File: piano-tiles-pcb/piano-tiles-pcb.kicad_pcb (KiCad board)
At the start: 2 copper layers, 72 x 52 mm, 18 parts, among them J1 Conn_01x05, J2 Conn_01x05, SW1 SW_SPST, SW2 SW_SPST, SW3 SW_SPST, SW4 SW_SPST, SW5 SW_SPDT

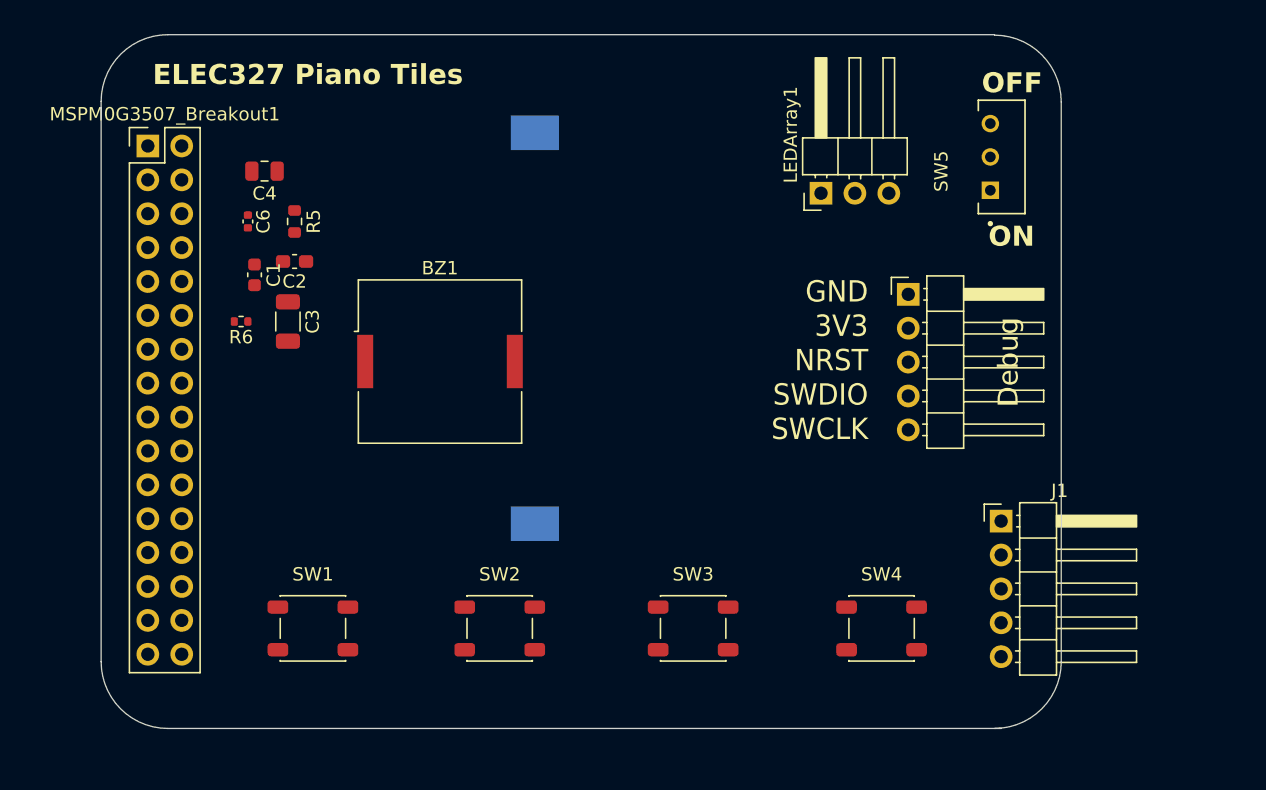
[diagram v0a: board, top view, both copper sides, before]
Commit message: first order
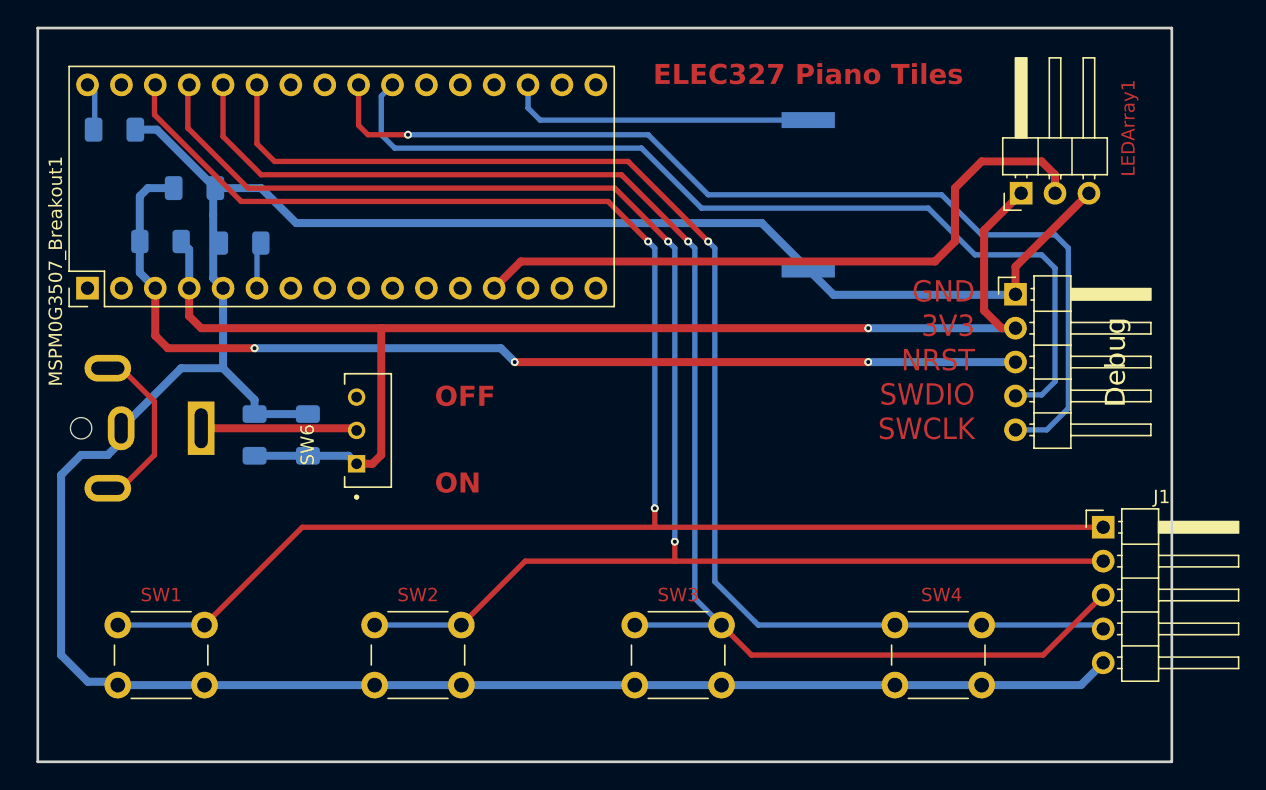
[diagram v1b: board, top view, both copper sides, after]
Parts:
- removed BT1: Battery_Cell, Battery:BatteryHolder_Keystone_1060_1x2032
- removed C3: 100uF, Capacitor_SMD:C_1206_3216Metric
- removed SW5: SW_SPDT, ELEC327-Kicad:SW_EG1270
- added J3: Barrel_Jack_MountingPin, Connector_BarrelJack:BarrelJack_CUI_PJ-063AH_Horizontal, B.Cu at (117.5, 106.5)
- added SW6: SW_SPDT, ELEC327-Kicad:SW_EG1270, F.Cu at (129.2, 106.7)
- BZ1: moved to B.Cu
- C1: footprint Capacitor_SMD:C_0603_1608Metric -> Capacitor_SMD:C_1206_3216Metric_Pad1.33x1.80mm_HandSolder; moved to B.Cu
- C2: footprint Capacitor_SMD:C_0603_1608Metric_Pad1.08x0.95mm_HandSolder -> Capacitor_SMD:C_1206_3216Metric_Pad1.33x1.80mm_HandSolder; moved to B.Cu
- C4: footprint Capacitor_SMD:C_0805_2012Metric -> Capacitor_SMD:C_1206_3216Metric_Pad1.33x1.80mm_HandSolder; moved to B.Cu
- C6: footprint Capacitor_SMD:C_0402_1005Metric -> Capacitor_SMD:C_1206_3216Metric_Pad1.33x1.80mm_HandSolder; moved to B.Cu
- MSPM0G3507_Breakout1: footprint Connector_PinHeader_2.54mm:PinHeader_2x16_P2.54mm_Vertical -> ELEC327-Kicad:QFN32Breakout-PinHeader_2x16_P2.54mm_Vertical
- R5: footprint Resistor_SMD:R_0603_1608Metric -> Resistor_SMD:R_1206_3216Metric_Pad1.30x1.75mm_HandSolder; moved to B.Cu
- R6: footprint Resistor_SMD:R_0402_1005Metric -> Resistor_SMD:R_1206_3216Metric_Pad1.30x1.75mm_HandSolder; moved to B.Cu
- SW1, SW2, SW3, SW4: footprint Button_Switch_SMD:SW_SPST_PTS647_Sx38 -> Button_Switch_THT:SW_PUSH_6mm_H5mm
- moved BZ1 30.3 mm to (163.0, 89.0), turned to -90 degrees
- moved LEDArray1 15.0 mm to (179.0, 88.9)
- moved SW1 14.6 mm to (111.2, 121.2)
- moved C2 13.0 mm to (125.5, 107.0), turned to 90 degrees
- moved C1 12.0 mm to (121.5, 107.0), turned to 90 degrees
- moved C4 11.7 mm to (111.0, 84.1), turned to 0 degrees
- moved MSPM0G3507_Breakout1 11.6 mm to (109.0, 96.0), turned to 90 degrees
- moved R5 10.2 mm to (114.5, 92.5), turned to 0 degrees
- moved SW2 9.38 mm to (130.5, 121.2)
- moved J2 8.04 mm to (178.5, 96.5)
- moved J1 7.66 mm to (185.1, 113.9)
- moved R6 5.88 mm to (120.4, 92.6), turned to 0 degrees
- moved C6 4.72 mm to (117.0, 88.5), turned to 0 degrees
- moved SW3 4.38 mm to (150.0, 121.2)
- moved SW4 1.03 mm to (169.5, 121.2)
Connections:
- J1 pad 1: GND -> BUTTON1_IO
- J1 pad 2: BUTTON4_IO -> BUTTON2_IO
- J1 pad 4: BUTTON2_IO -> BUTTON4_IO
- J1 pad 5: BUTTON1_IO -> GND
- MSPM0G3507_Breakout1 pad 16: ACC_INT -> unconnected-(MSPM0G3507_Breakout1-Pin_16-Pad16)
- MSPM0G3507_Breakout1 pad 23: unconnected-(MSPM0G3507_Breakout1-Pin_23-Pad23) -> SWDIO
- MSPM0G3507_Breakout1 pad 24: unconnected-(MSPM0G3507_Breakout1-Pin_24-Pad24) -> SWCLK
- MSPM0G3507_Breakout1 pad 27: BUTTON1_IO -> BUTTON4_IO
- MSPM0G3507_Breakout1 pad 28: BUTTON2_IO -> BUTTON3_IO
- MSPM0G3507_Breakout1 pad 29: BUTTON3_IO -> BUTTON2_IO
- MSPM0G3507_Breakout1 pad 30: BUTTON4_IO -> BUTTON1_IO
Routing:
- net GND: track 0.00 -> 212.9 mm
- net BUTTON1_IO: track 0.00 -> 141.7 mm, vias 0 -> 2
- net BUTTON2_IO: track 0.00 -> 123.6 mm, vias 0 -> 2
- net BUTTON3_IO: track 0.00 -> 109.7 mm, vias 0 -> 1
- net VDD: track 0.00 -> 100.5 mm, vias 0 -> 1
- net BUTTON4_IO: track 0.00 -> 97.6 mm, vias 0 -> 1
- net NRST: track 0.00 -> 79.0 mm, vias 0 -> 3
- net SWCLK: track 0.00 -> 76.7 mm, vias 0 -> 1
- net SWDIO: track 0.00 -> 70.6 mm
- net SPI0_LED_PICO: track 0.00 -> 50.1 mm
- net BUZZER_IO: track 0.00 -> 23.1 mm
- net unconnected-(J3-MountPin-PadMP): track 0.00 -> 13.1 mm
- net Net-(SW6-B): track 0.00 -> 11.7 mm
- net VCORE: track 0.00 -> 3.58 mm
- net ROSC: track 0.00 -> 3.50 mm
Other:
- board size 72 x 52 mm -> 85 x 55 mm
